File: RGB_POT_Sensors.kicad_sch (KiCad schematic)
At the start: 14 parts, among them J10 RGB, J7 LM_35, J8 LDR, J9 POT, U6 LM35-LP

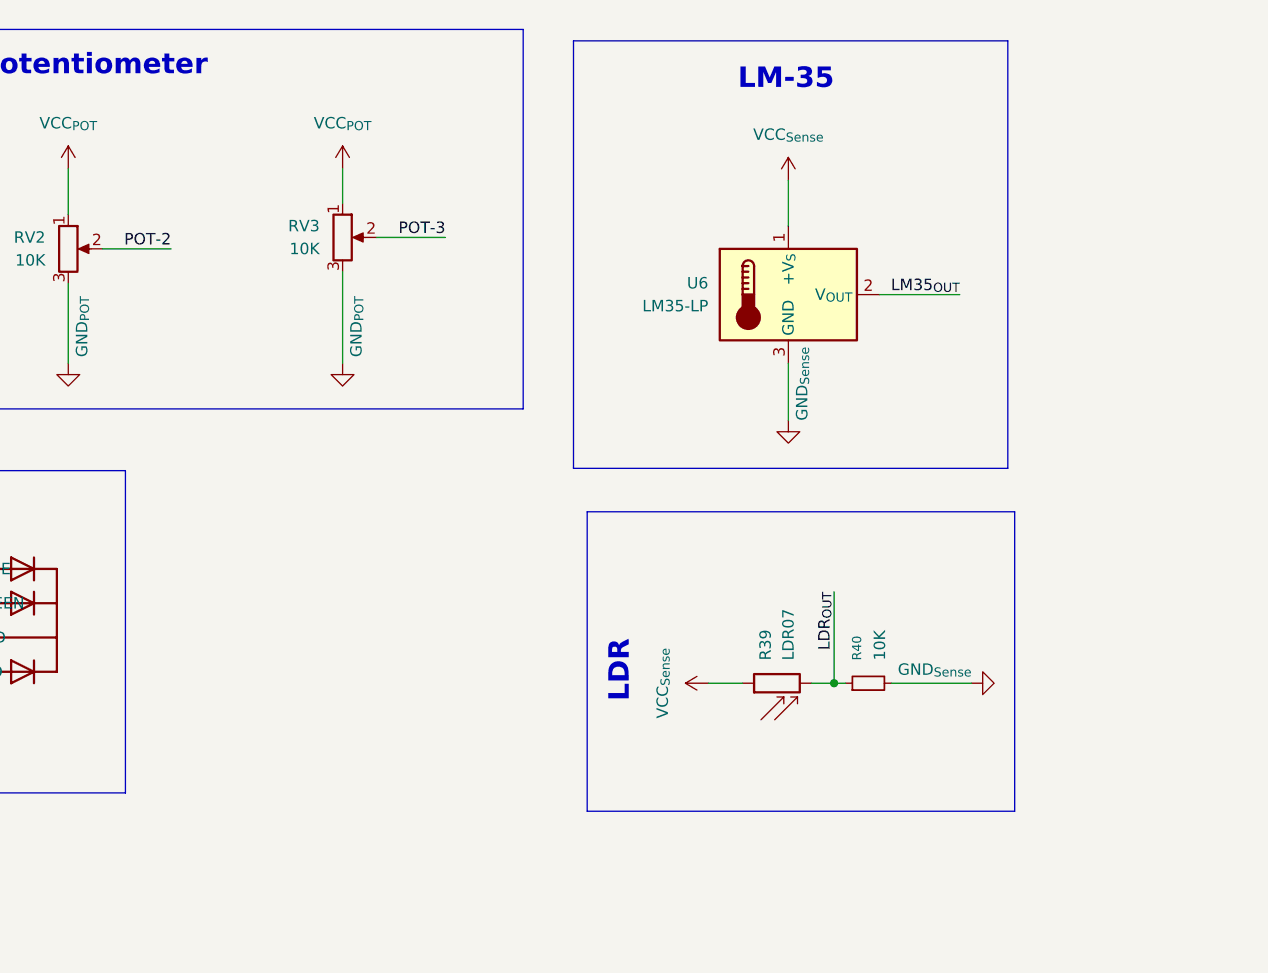
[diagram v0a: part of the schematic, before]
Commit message: Schematic Completed, Footprints Assigned
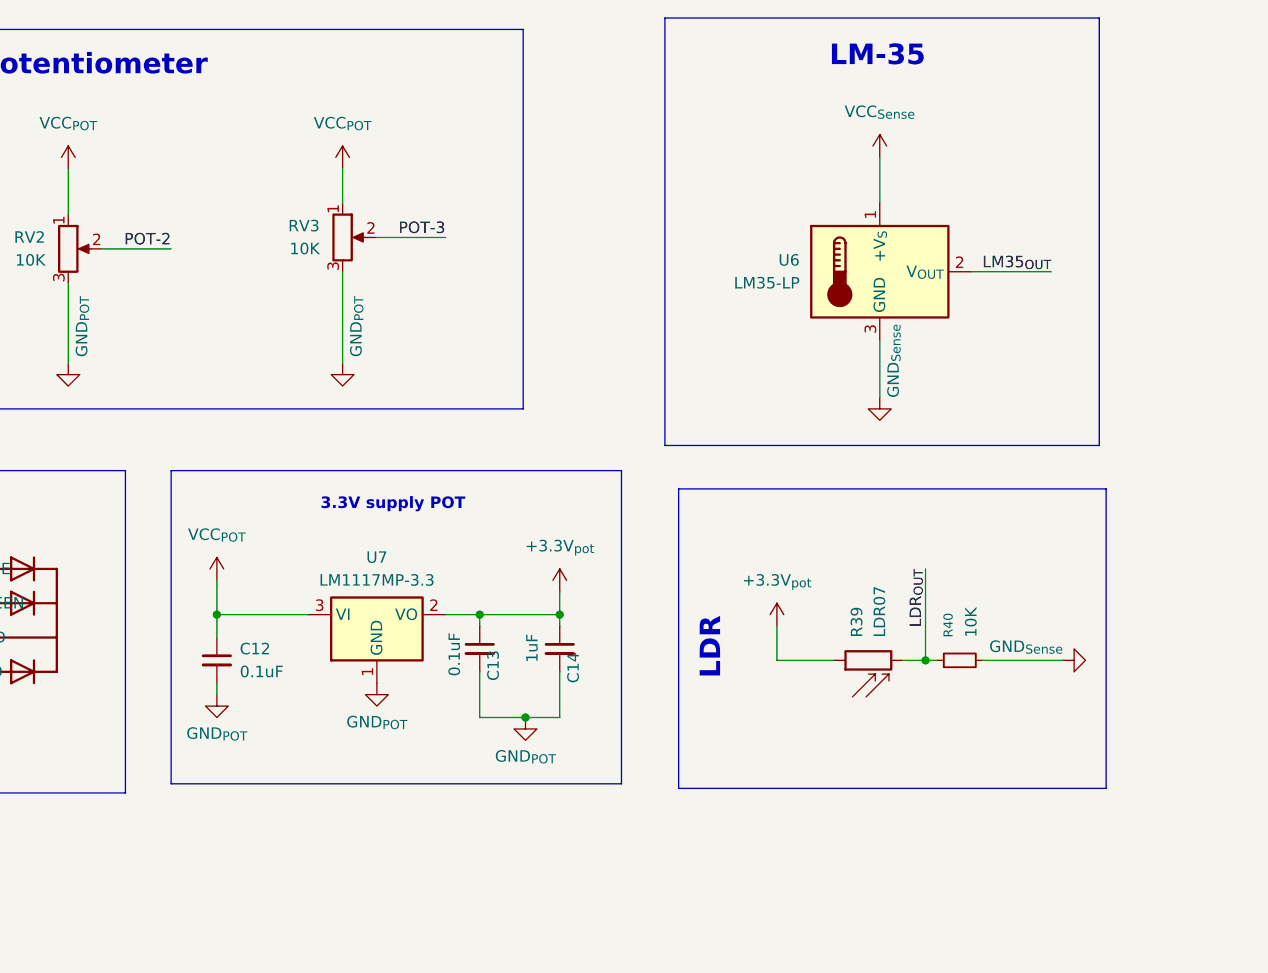
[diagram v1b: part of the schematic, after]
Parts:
- added C12, C13: 0.1uF, Capacitor_SMD:C_0805_2012Metric_Pad1.18x1.45mm_HandSolder, symbol Device:C_Small
- added C14: 1uF, Capacitor_SMD:C_0805_2012Metric_Pad1.18x1.45mm_HandSolder, symbol Device:C_Small
- added U7: LM1117MP-3.3, Package_TO_SOT_SMD:SOT-223-3_TabPin2, symbol Regulator_Linear:LM1117MP-3.3
- J10, J9: footprint (none) -> Connector_JST:JST_EH_B5B-EH-A_1x05_P2.50mm_Vertical
- J7, J8: footprint (none) -> Connector_JST:JST_EH_B3B-EH-A_1x03_P2.50mm_Vertical
- R36, R37, R38, R40: footprint (none) -> Resistor_SMD:R_0805_2012Metric_Pad1.20x1.40mm_HandSolder
- RV1, RV2, RV3: footprint (none) -> LOGSUN:LGS-KC-CA6V
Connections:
- net GND_{POT}: now also C12.2, C13.2, C14.2, U7.1 (GND)
- net VCC_{POT}: now also C12.1, U7.3 (VI)
- net VCC_{Sense}: no longer R39.1
- new net +3.3V_{pot}: C13.1, C14.1, R39.1, U7.2 (VO)
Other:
- note added: "3.3V supply POT"
- moved on the sheet: R39, R40, U6

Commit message: Symbol and footprint library exported
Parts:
- C12, C13, C14: symbol Device:C_Small -> ESP32_Xbee_LoRa:C_Small
- D19: symbol LOGSUN:LGS-KC-5MMRGBLED -> ESP32_Xbee_LoRa:LGS-KC-5MMRGBLED
- J10, J9: symbol Connector:Conn_01x05_Pin -> ESP32_Xbee_LoRa:Conn_01x05_Pin
- J7, J8: symbol Connector:Conn_01x03_Pin -> ESP32_Xbee_LoRa:Conn_01x03_Pin
- R36, R37, R38, R40: symbol Device:R_Small -> ESP32_Xbee_LoRa:R_Small
- R39: symbol Sensor_Optical:LDR07 -> ESP32_Xbee_LoRa:LDR07
- RV1, RV2, RV3: symbol Device:R_Potentiometer -> ESP32_Xbee_LoRa:R_Potentiometer
- U6: symbol Sensor_Temperature:LM35-LP -> ESP32_Xbee_LoRa:LM35-LP
- U7: symbol Regulator_Linear:LM1117MP-3.3 -> ESP32_Xbee_LoRa:LM1117MP-3.3
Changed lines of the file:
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@@
 	)
 	(symbol
-		(lib_id "Device:R_Small")
+		(lib_id "ESP32_Xbee_LoRa:R_Small")
 		(at 31.75 80.01 90)
 		(unit 1)
@@
 	)
 	(symbol
-		(lib_id "Device:C_Small")
+		(lib_id "ESP32_Xbee_LoRa:C_Small")
 		(at 107.95 88.9 0)
 		(unit 1)
@@
 	)
 	(symbol
-		(lib_id "Sensor_Optical:LDR07")
+		(lib_id "ESP32_Xbee_LoRa:LDR07")
 		(at 151.13 90.17 90)
 		(unit 1)
@@
 	)
 	(symbol
-		(lib_id "power:GND")
+		(lib_id "ESP32_Xbee_LoRa:GND")
 		(at 92.71 57.15 0)
 		(unit 1)
@@
 	)
 	(symbol
-		(lib_id "power:GND")
+		(lib_id "ESP32_Xbee_LoRa:GND")
 		(at 172.72 90.17 90)
 		(unit 1)
@@
 	)
 	(symbol
-		(lib_id "Device:R_Small")
+		(lib_id "ESP32_Xbee_LoRa:R_Small")
 		(at 31.75 91.44 90)
 		(unit 1)
@@
 	)
 	(symbol
-		(lib_id "power:VCC")
+		(lib_id "ESP32_Xbee_LoRa:VCC")
 		(at 78.74 81.28 0)
 		(unit 1)
@@
 	)
 	(symbol
-		(lib_id "power:VCC")
+		(lib_id "ESP32_Xbee_LoRa:VCC")
 		(at 228.6 41.91 0)
 		(unit 1)
@@
 	)
 	(symbol
-		(lib_id "power:GND")
+		(lib_id "ESP32_Xbee_LoRa:GND")
 		(at 152.4 60.96 0)
 		(unit 1)
@@
 	)
 	(symbol
-		(lib_id "power:VCC")
+		(lib_id "ESP32_Xbee_LoRa:VCC")
 		(at 256.54 76.2 0)
 		(unit 1)
@@
 	)
 	(symbol
-		(lib_id "Connector:Conn_01x03_Pin")
+		(lib_id "ESP32_Xbee_LoRa:Conn_01x03_Pin")
 		(at 248.92 48.26 0)
 		(unit 1)
@@
 	)
 	(symbol
-		(lib_id "power:GND")
+		(lib_id "ESP32_Xbee_LoRa:GND")
 		(at 96.52 92.71 0)
 		(unit 1)
@@
 	)
 	(symbol
-		(lib_id "Connector:Conn_01x05_Pin")
+		(lib_id "ESP32_Xbee_LoRa:Conn_01x05_Pin")
 		(at 248.92 83.82 0)
 		(unit 1)
@@
 	)
 	(symbol
-		(lib_id "Regulator_Linear:LM1117MP-3.3")
+		(lib_id "ESP32_Xbee_LoRa:LM1117MP-3.3")
 		(at 96.52 85.09 0)
 		(unit 1)
@@
 	)
 	(symbol
-		(lib_id "power:VCC")
+		(lib_id "ESP32_Xbee_LoRa:VCC")
 		(at 62.23 35.56 0)
 		(unit 1)
@@
 	)
 	(symbol
-		(lib_id "Device:R_Potentiometer")
+		(lib_id "ESP32_Xbee_LoRa:R_Potentiometer")
 		(at 31.75 45.72 0)
 		(unit 1)
@@
 	)
 	(symbol
-		(lib_id "power:VCC")
+		(lib_id "ESP32_Xbee_LoRa:VCC")
 		(at 152.4 34.29 0)
 		(unit 1)
@@
 	)
 	(symbol
-		(lib_id "Device:R_Potentiometer")
+		(lib_id "ESP32_Xbee_LoRa:R_Potentiometer")
 		(at 92.71 43.18 0)
 		(unit 1)
@@
 	)
 	(symbol
-		(lib_id "Connector:Conn_01x03_Pin")
+		(lib_id "ESP32_Xbee_LoRa:Conn_01x03_Pin")
 		(at 219.71 48.26 0)
 		(unit 1)
@@
 	)
 	(symbol
-		(lib_id "power:VCC")
+		(lib_id "ESP32_Xbee_LoRa:VCC")
 		(at 92.71 35.56 0)
 		(unit 1)
@@
 	)
 	(symbol
-		(lib_id "power:GND")
+		(lib_id "ESP32_Xbee_LoRa:GND")
 		(at 228.6 53.34 0)
 		(unit 1)
@@
 	)
 	(symbol
-		(lib_id "LOGSUN:LGS-KC-5MMRGBLED")
+		(lib_id "ESP32_Xbee_LoRa:LGS-KC-5MMRGBLED")
 		(at 60.96 87.63 270)
 		(unit 1)
@@
 	)
 	(symbol
-		(lib_id "Device:C_Small")
+		(lib_id "ESP32_Xbee_LoRa:C_Small")
 		(at 78.74 90.17 0)
 		(unit 1)
@@
 	)
 	(symbol
-		(lib_id "power:+3.3V")
+		(lib_id "ESP32_Xbee_LoRa:+3.3V")
 		(at 116.84 82.55 0)
 		(unit 1)
@@
 	)
 	(symbol
-		(lib_id "Connector:Conn_01x05_Pin")
+		(lib_id "ESP32_Xbee_LoRa:Conn_01x05_Pin")
 		(at 223.52 82.55 0)
 		(unit 1)
@@
 	)
 	(symbol
-		(lib_id "power:GND")
+		(lib_id "ESP32_Xbee_LoRa:GND")
 		(at 62.23 57.15 0)
 		(unit 1)
@@
 	)
 	(symbol
-		(lib_id "Device:R_Small")
+		(lib_id "ESP32_Xbee_LoRa:R_Small")
 		(at 39.37 83.82 90)
 		(unit 1)
@@
 	)
 	(symbol
-		(lib_id "power:GND")
+		(lib_id "ESP32_Xbee_LoRa:GND")
 		(at 41.91 100.33 0)
 		(unit 1)
@@
 	)
 	(symbol
-		(lib_id "Logsun_Logo:LOGO")
+		(lib_id "ESP32_Xbee_LoRa:LOGO")
 		(at 259.08 173.99 0)
 		(unit 1)
@@
 	)
 	(symbol
-		(lib_id "power:GND")
+		(lib_id "ESP32_Xbee_LoRa:GND")
 		(at 31.75 57.15 0)
 		(unit 1)
@@
 	)
 	(symbol
-		(lib_id "power:VCC")
+		(lib_id "ESP32_Xbee_LoRa:VCC")
 		(at 257.81 41.91 0)
 		(unit 1)
@@
 	)
 	(symbol
-		(lib_id "Device:C_Small")
+		(lib_id "ESP32_Xbee_LoRa:C_Small")
 		(at 116.84 88.9 0)
 		(unit 1)
@@
 	)
 	(symbol
-		(lib_id "power:GND")
+		(lib_id "ESP32_Xbee_LoRa:GND")
 		(at 78.74 93.98 0)
 		(unit 1)
@@
 	)
 	(symbol
-		(lib_id "power:+3.3V")
+		(lib_id "ESP32_Xbee_LoRa:+3.3V")
 		(at 140.97 86.36 0)
 		(unit 1)
@@
 	)
 	(symbol
-		(lib_id "Device:R_Small")
+		(lib_id "ESP32_Xbee_LoRa:R_Small")
 		(at 161.29 90.17 90)
 		(unit 1)
@@
 	)
 	(symbol
-		(lib_id "Sensor_Temperature:LM35-LP")
+		(lib_id "ESP32_Xbee_LoRa:LM35-LP")
 		(at 152.4 46.99 0)
 		(unit 1)
@@
 	)
 	(symbol
-		(lib_id "power:GND")
+		(lib_id "ESP32_Xbee_LoRa:GND")
 		(at 232.41 90.17 0)
 		(unit 1)
@@
 	)
 	(symbol
-		(lib_id "Device:R_Potentiometer")
+		(lib_id "ESP32_Xbee_LoRa:R_Potentiometer")
 		(at 62.23 44.45 0)
 		(unit 1)
@@
 	)
 	(symbol
-		(lib_id "power:GND")
+		(lib_id "ESP32_Xbee_LoRa:GND")
 		(at 113.03 96.52 0)
 		(unit 1)
@@
 	)
 	(symbol
-		(lib_id "power:GND")
+		(lib_id "ESP32_Xbee_LoRa:GND")
 		(at 256.54 91.44 0)
 		(unit 1)
@@
 	)
 	(symbol
-		(lib_id "power:GND")
+		(lib_id "ESP32_Xbee_LoRa:GND")
 		(at 257.81 53.34 0)
 		(unit 1)
@@
 	)
 	(symbol
-		(lib_id "power:VCC")
+		(lib_id "ESP32_Xbee_LoRa:VCC")
 		(at 31.75 35.56 0)
 		(unit 1)
